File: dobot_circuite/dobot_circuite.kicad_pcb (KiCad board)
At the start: 2 copper layers, 146 x 146 mm, 29 parts, among them J1 USB_A, J2 USB_A, J3 USB_A, J4 USB_A, J5 USB_A, J6 USB_A, J7 HDMI, J8 Jack-DC, J9 HDMI, U1 FE1.1s, U2 FE1.1s, U3 usb_connector, U4 XH_DCJ, U5 usb_connector, U6 HDMI_Hole, U7 HDMI_Hole2, U8 arduino_leonard, Y1 Crystal, Y2 Crystal

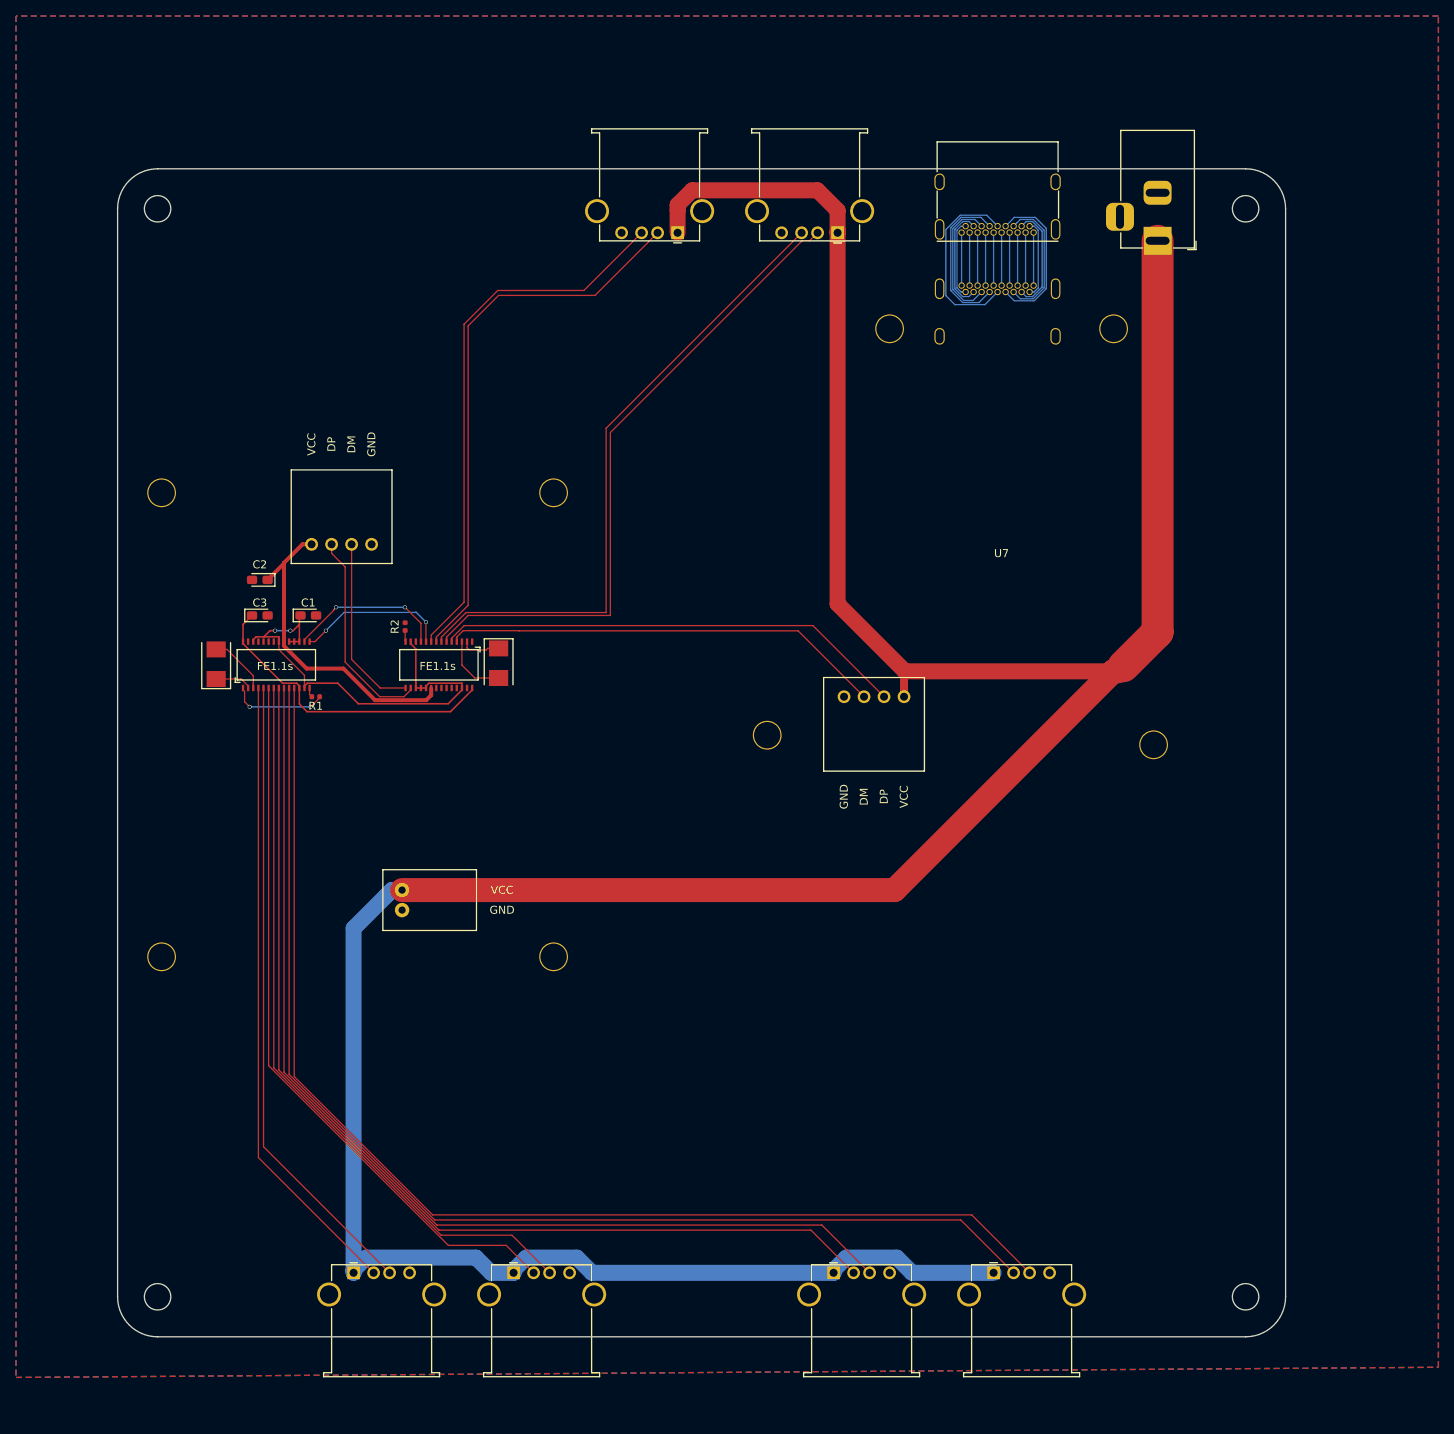
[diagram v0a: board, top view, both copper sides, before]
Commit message: Add files via upload
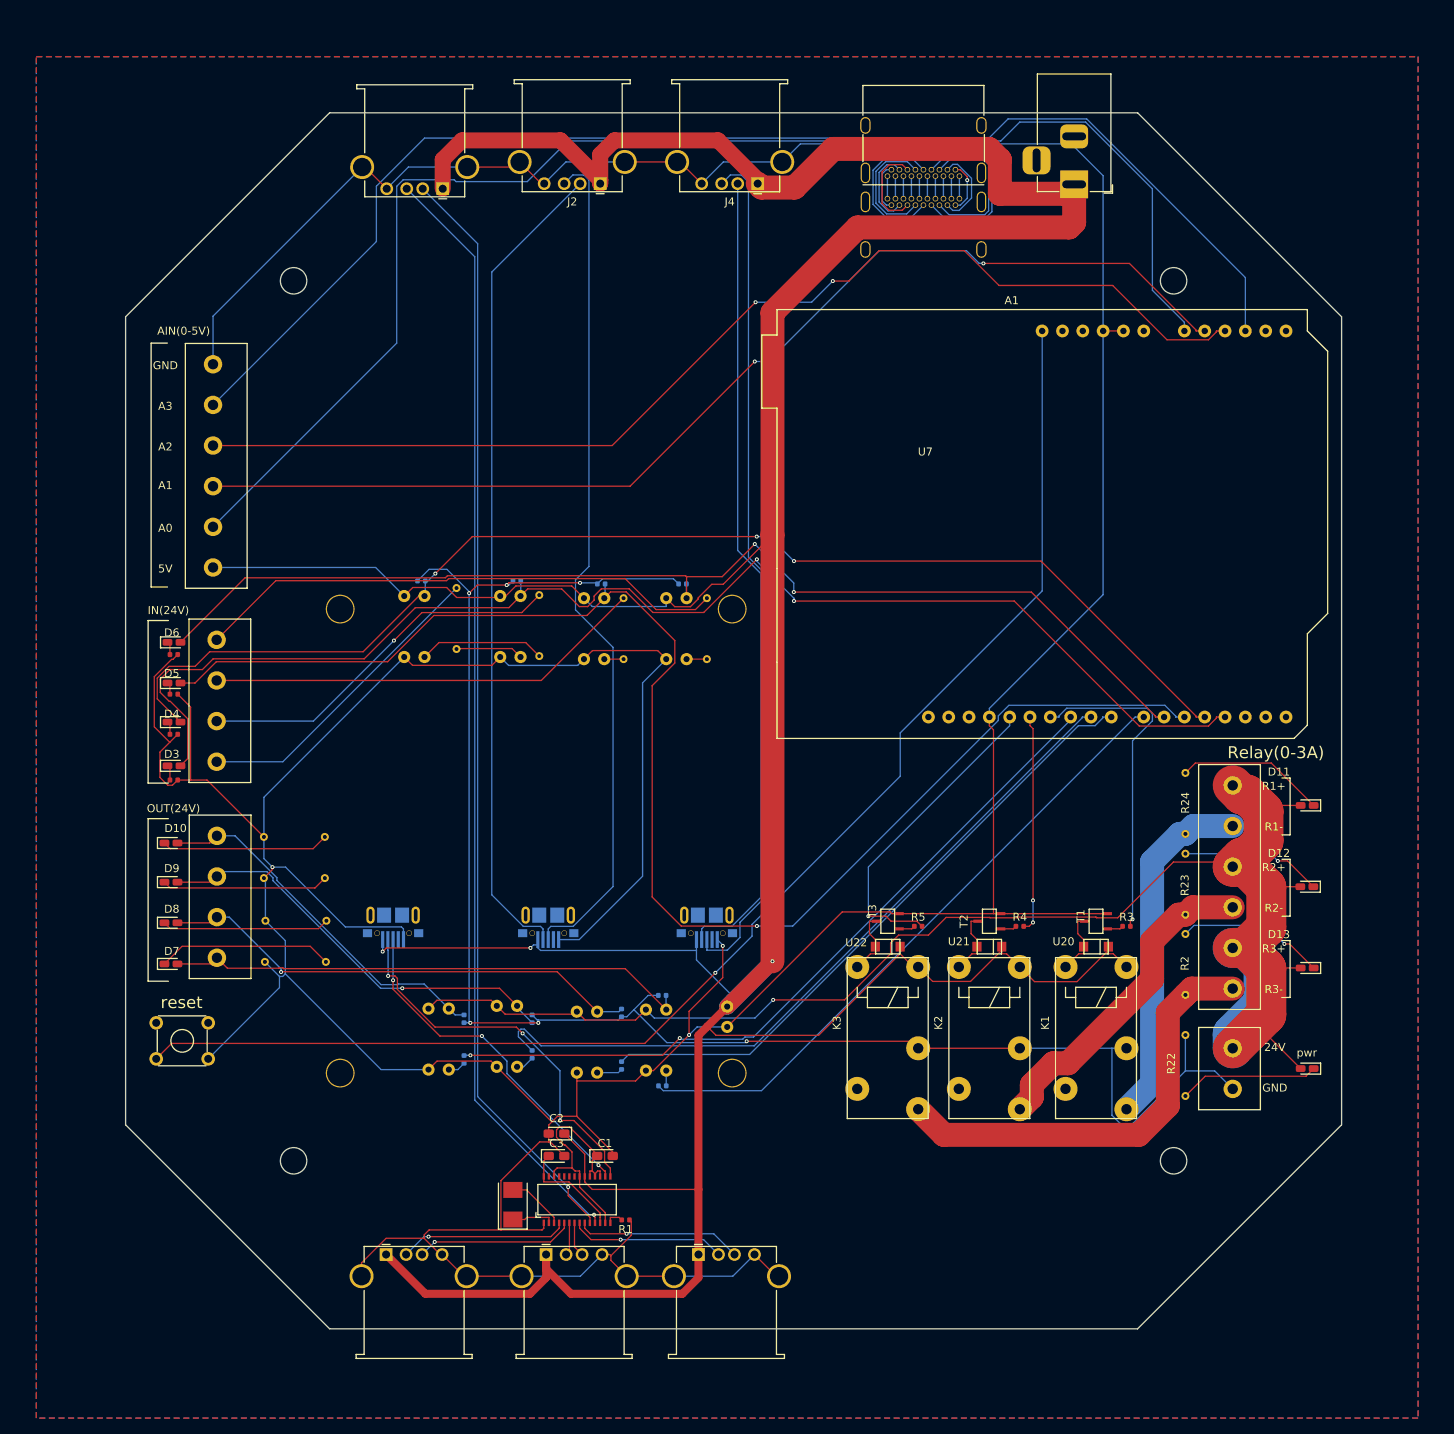
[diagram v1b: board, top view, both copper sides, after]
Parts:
- removed U4: XH_DCJ, hoshina_library:S2B-XH-A_DCJ
- removed U6: HDMI_Hole, hoshina_library:HDMI_Hole
- removed Y2: Crystal, hoshina_library:Crystal_SMD_5032-2Pin_5.0x3.2mm
- added A1: Arduino_Leonardo_pin_remove_2pin, hoshina_library:arduino_leonard_remove_2pin, F.Cu at (110.5, -125.7)
- added D1: LED_green, hoshina_library:LED_1608, F.Cu at (148.7, -33.5)
- added K1: ALQ105, hoshina_library:ALQ105_akituki, F.Cu at (126.1, -46.2)
- added K2: ALQ105, hoshina_library:ALQ105_akituki, F.Cu at (112.8, -46.2)
- added K3: ALQ105, hoshina_library:ALQ105_akituki, F.Cu at (100.1, -46.2)
- added R10: 10k, hoshina_library:register_0603, B.Cu at (49.9, -94.5)
- added R11: 10k, hoshina_library:register_0603, B.Cu at (60.5, -94.1)
- added R12: 1k/1W, hoshina_library:carbon_register, B.Cu at (52.7, -85.1)
- added R13: 1k/1W, hoshina_library:carbon_register, B.Cu at (73.7, -84.7)
- added R14: 10k, hoshina_library:register_0603, B.Cu at (38.0, -94.5)
- added R15: 10k, hoshina_library:register_0603, B.Cu at (70.6, -94.1)
- added R16: 190, hoshina_library:register_0603, B.Cu at (68.1, -31.4)
- added R17: 190, hoshina_library:register_0603, B.Cu at (51.8, -35.3)
- added R18: 10k, hoshina_library:register_0603, B.Cu at (68.1, -42.7)
- added R19: 10k, hoshina_library:register_0603, B.Cu at (51.8, -39.8)
- added R20: 190, hoshina_library:register_0603, B.Cu at (63.0, -33.9)
- added R21: 10k, hoshina_library:register_0603, B.Cu at (63.0, -40.5)
- added R22: R, hoshina_library:carbon_register, F.Cu at (133.5, -30.1)
- added R23: 5.6k/1w, hoshina_library:carbon_register, F.Cu at (133.5, -60.4)
- added R24: 5.6k/1w, hoshina_library:carbon_register, F.Cu at (133.5, -70.5)
- added R25: 4.7k, hoshina_library:register_0603, F.Cu at (7.03, -75.3)
- added R26: 4.7k, hoshina_library:register_0603, F.Cu at (7.03, -69.6)
- added R27: 4.7k, hoshina_library:register_0603, F.Cu at (7.03, -80.3)
- added R28: 4.7k, hoshina_library:register_0603, F.Cu at (7.03, -85.3)
- added R29: 5.6k/1w, hoshina_library:carbon_register, B.Cu at (26.0, -46.9)
- added R3: 5k, hoshina_library:register_0603, F.Cu at (126.1, -51.3)
- added R30: 5.6k/1w, hoshina_library:carbon_register, B.Cu at (26.1, -52.0)
- added R31: 5.6k/1w, hoshina_library:carbon_register, B.Cu at (25.9, -57.3)
- added R32: 5.6k/1w, hoshina_library:carbon_register, B.Cu at (25.9, -62.5)
- added R4: 5k, hoshina_library:register_0603, F.Cu at (112.8, -51.3)
- added R5: 5k, hoshina_library:register_0603, F.Cu at (100.1, -51.3)
- added R6: 190, hoshina_library:register_0603, B.Cu at (43.3, -34.7)
- added R7: 10k, hoshina_library:register_0603, B.Cu at (43.3, -39.8)
- added R8: 1k/1W, hoshina_library:carbon_register, B.Cu at (42.4, -86.0)
- added R9: 1k/1W, hoshina_library:carbon_register, B.Cu at (63.2, -84.7)
- added SW1: SW_Push_Dual, hoshina_library:SW_TH_Tactile_Omron_B3F-10xx, F.Cu at (4.83, -39.2)
- added T1: 2SD1781K, hoshina_library:2SD1781, F.Cu at (122.3, -51.9)
- added T2: 2SD1781K, hoshina_library:2SD1781, F.Cu at (109.0, -51.9)
- added T3: 2SD1781K, hoshina_library:2SD1781, F.Cu at (96.3, -51.9)
- added U10: fhoto_capura_PS817, hoshina_library:fhoto_capra_PS817, B.Cu at (41.4, -33.4)
- added U11: terminal_block_4pin_small, hoshina_library:terminal_block_4pin_small, F.Cu at (12.4, -62.6)
- added U12: fhoto_capura_PS817, hoshina_library:fhoto_capra_PS817, B.Cu at (50.4, -85.0)
- added U13: fhoto_capura_PS817, hoshina_library:fhoto_capra_PS817, B.Cu at (60.8, -84.7)
- added U14: fhoto_capura_PS817, hoshina_library:fhoto_capra_PS817, B.Cu at (38.4, -85.0)
- added U15: fhoto_capura_PS817, hoshina_library:fhoto_capra_PS817, B.Cu at (71.1, -84.7)
- added U16: terminal_block_4pin_small, hoshina_library:terminal_block_4pin_small, F.Cu at (12.4, -87.1)
- added U17: fhoto_capura_PS817, hoshina_library:fhoto_capra_PS817, B.Cu at (68.6, -33.3)
- added U18: fhoto_capura_PS817, hoshina_library:fhoto_capra_PS817, B.Cu at (49.9, -33.7)
- added U19: fhoto_capura_PS817, hoshina_library:fhoto_capra_PS817, B.Cu at (59.9, -33.0)
- added U20: diode_GS1010FL, hoshina_library:diode_GS1010FL, F.Cu at (122.3, -48.8)
- added U21: diode_GS1010FL, hoshina_library:diode_GS1010FL, F.Cu at (109.0, -48.8)
- added U22: diode_GS1010FL, hoshina_library:diode_GS1010FL, F.Cu at (96.3, -48.8)
- added U23: terminal_block_6pin_small, hoshina_library:terminal_block_6pin_small, F.Cu at (11.9, -121.6)
- added U9: terminal_block_2pin_small, hoshina_library:terminal_block_2pin_small, F.Cu at (139.4, -33.5)
- added hand_electric_line1: hoshina_library_terminal_block_2pin_small, hoshina_library:2pin_power_gnd, F.Cu at (76.2, -41.3)
- added led1: LED, hoshina_library:LED_1608, F.Cu at (148.7, -46.1)
- added led10: LED, hoshina_library:LED_1608, F.Cu at (6.67, -56.8)
- added led11: LED, hoshina_library:LED_1608, F.Cu at (6.67, -61.7)
- added led2: LED, hoshina_library:LED_1608, F.Cu at (148.7, -56.3)
- added led3: LED, hoshina_library:LED_1608, F.Cu at (148.7, -66.4)
- added led4: LED, hoshina_library:LED_1608, F.Cu at (7.05, -76.8)
- added led5: LED, hoshina_library:LED_1608, F.Cu at (7.05, -71.4)
- added led6: LED, hoshina_library:LED_1608, F.Cu at (7.05, -81.7)
- added led7: LED, hoshina_library:LED_1608, F.Cu at (7.05, -86.8)
- added led8: LED, hoshina_library:LED_1608, F.Cu at (6.67, -46.6)
- added led9: LED, hoshina_library:LED_1608, F.Cu at (6.67, -51.8)
- R2: value R -> 5.6k/1w; footprint hoshina_library:register_0603 -> hoshina_library:carbon_register
- U2: value FE1.1s -> microB_usb_connector; footprint hoshina_library:FE1.1s -> hoshina_library:USB_Micro-B_MC5F-03_aitendo_reverse
- U3, U5: value usb_connector -> microB_usb_connector; footprint hoshina_library:XH4PIN_S -> hoshina_library:USB_Micro-B_MC5F-03_aitendo_reverse
- U8: value arduino_leonard -> terminal_block_6pin_small; footprint hoshina_library:arduino_leonard -> hoshina_library:terminal_block_6pin_small
- moved H1 179.6 mm to (132.0, -132.0)
- moved J1 152.0 mm to (40.6, -143.5), turned to 180 degrees
- moved H3 120.2 mm to (22.0, -22.0)
- moved H4 119.3 mm to (22.0, -132.0)
- moved R2 104.8 mm to (133.5, -50.4)
- moved C2 78.5 mm to (54.9, -25.4)
- moved C1 77.1 mm to (60.9, -22.6)
- moved C3 77.1 mm to (54.9, -22.6)
- moved Y1 77.1 mm to (49.4, -16.5)
- moved U1 76.7 mm to (61.6, -17.1)
- moved R1 76.0 mm to (63.5, -14.6)
- moved U3 51.3 mm to (53.8, -52.7), turned to 0 degrees
- moved U5 32.2 mm to (73.7, -52.7)
- moved U2 31.3 mm to (34.4, -52.7), turned to 0 degrees
- moved Thinker_board1 26.6 mm to (52.3, -29.5)
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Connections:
- R2 pad 1: GND -> Net-(R2-Pad1)
- R2 pad 2: Net-(R2-Pad2) -> D13_relay
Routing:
- net GND: track 12.1 -> 698.6 mm, vias 2 -> 3
- net GNDA: track 0.00 -> 213.1 mm, vias 0 -> 6
- net +24V: track 0.00 -> 196.3 mm, vias 0 -> 1
- net D5: track 0.00 -> 184.6 mm, vias 0 -> 1
- net A0: track 0.00 -> 172.9 mm
- net Net-(A1-PadRESET): track 0.00 -> 171.5 mm, vias 0 -> 1
- net D3: track 0.00 -> 168.0 mm, vias 0 -> 2
- net A3: track 0.00 -> 162.8 mm
- net D4: track 0.00 -> 155.4 mm, vias 0 -> 3
- net D6: track 0.00 -> 142.3 mm, vias 0 -> 2
- net A2: track 0.00 -> 141.7 mm, vias 0 -> 2
- net A1: track 0.00 -> 140.4 mm, vias 0 -> 2
- net Net-(J6-Pad3): track 131.6 -> 20.8 mm, vias 0 -> 1
- net Net-(J6-Pad2): track 130.1 -> 19.4 mm, vias 0 -> 1
- net +5V: track 449.9 -> 549.2 mm, vias 0 -> 3
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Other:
- board size 146 x 146 mm -> 152 x 152 mm
- net class Default: clearance 0.1 -> 0.2
- rule trace_clearance: 0.1 -> 0.2
- rule trace_min: 0.125 -> 0.16
- board text added: "24V"
- board text added: "5V"
- board text added: "A0"
- board text added: "A1"
- board text added: "A2"
- board text added: "A3"
- board text added: "AIN(0-5V)"
- board text added: "D10"
- board text added: "D11"
- board text added: "D12"
- board text added: "D13"
- board text added: "D3"
- board text added: "D4"
- board text added: "D5"
- board text added: "D6"
- board text added: "D7"
- board text added: "D8"
- board text added: "D9"
- board text added: "GND"
- board text added: "IN(24V)"
- board text added: "OUT(24V)"
- board text added: "R1+"
- board text added: "R1-"
- board text added: "R2+"
- board text added: "R2-"
- board text added: "R3+"
- board text added: "R3-"
- board text added: "Relay(0-3A)"
- board text added: "pwr"
- board text added: "reset"
